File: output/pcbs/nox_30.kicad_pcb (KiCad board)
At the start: 2 copper layers, 111.1 x 91.5 mm, 46 parts

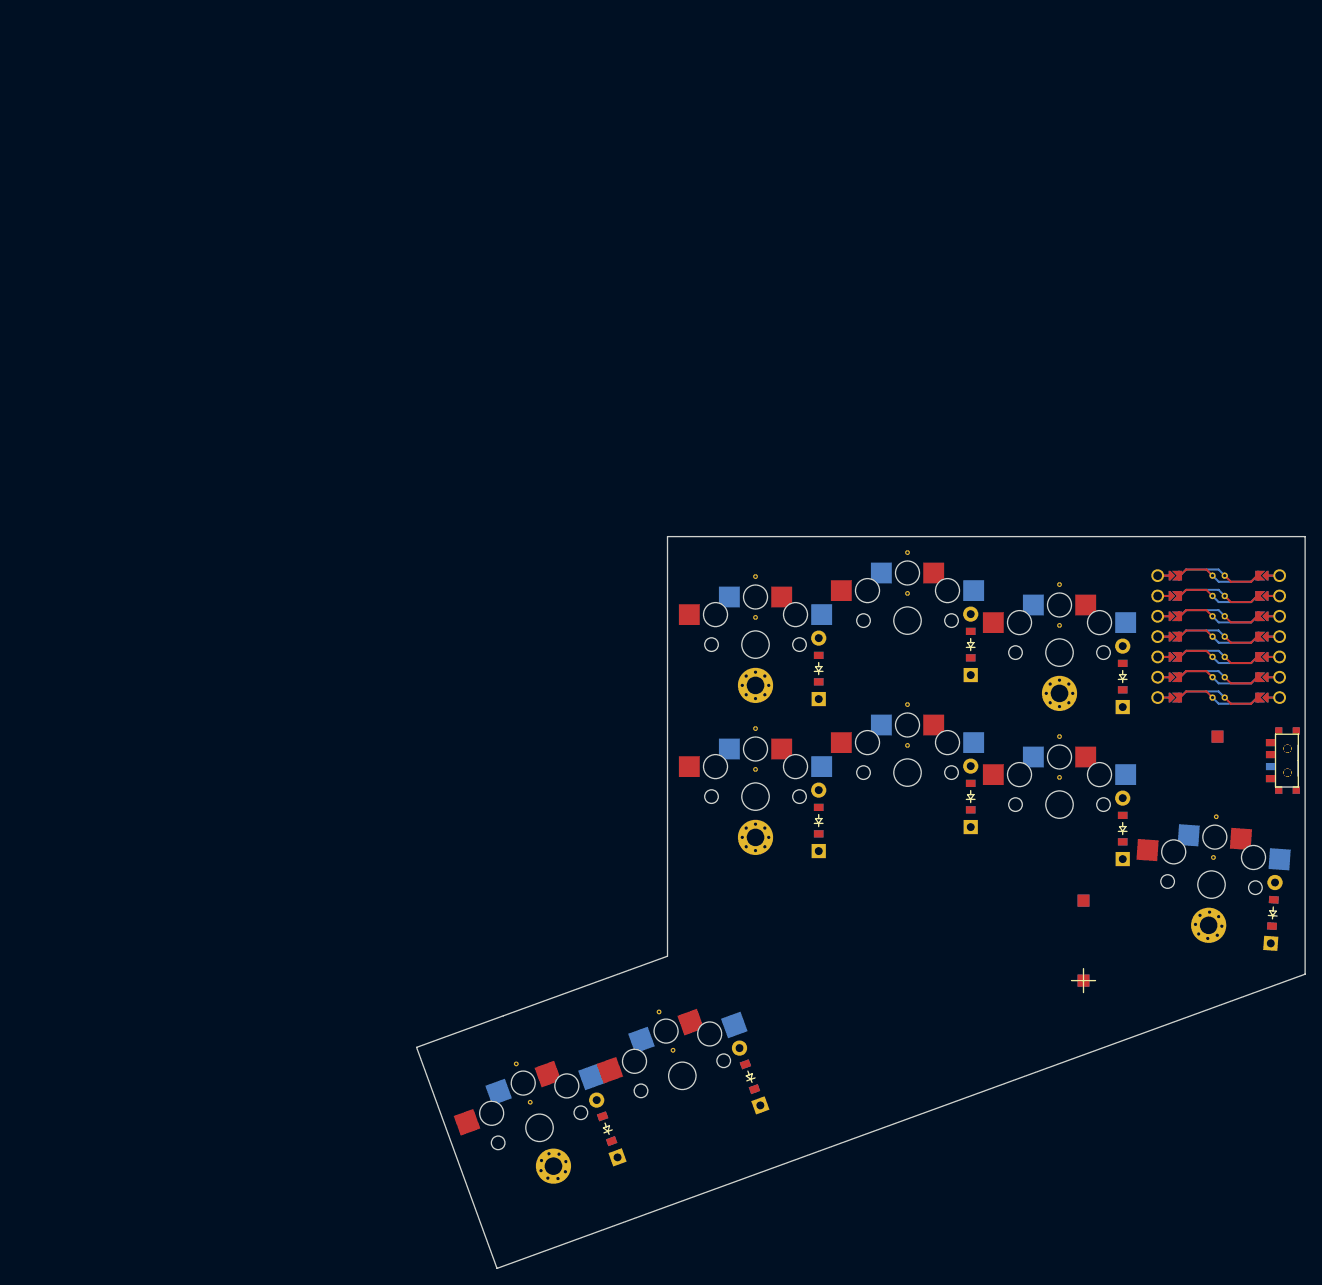
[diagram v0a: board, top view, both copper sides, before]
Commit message: update case
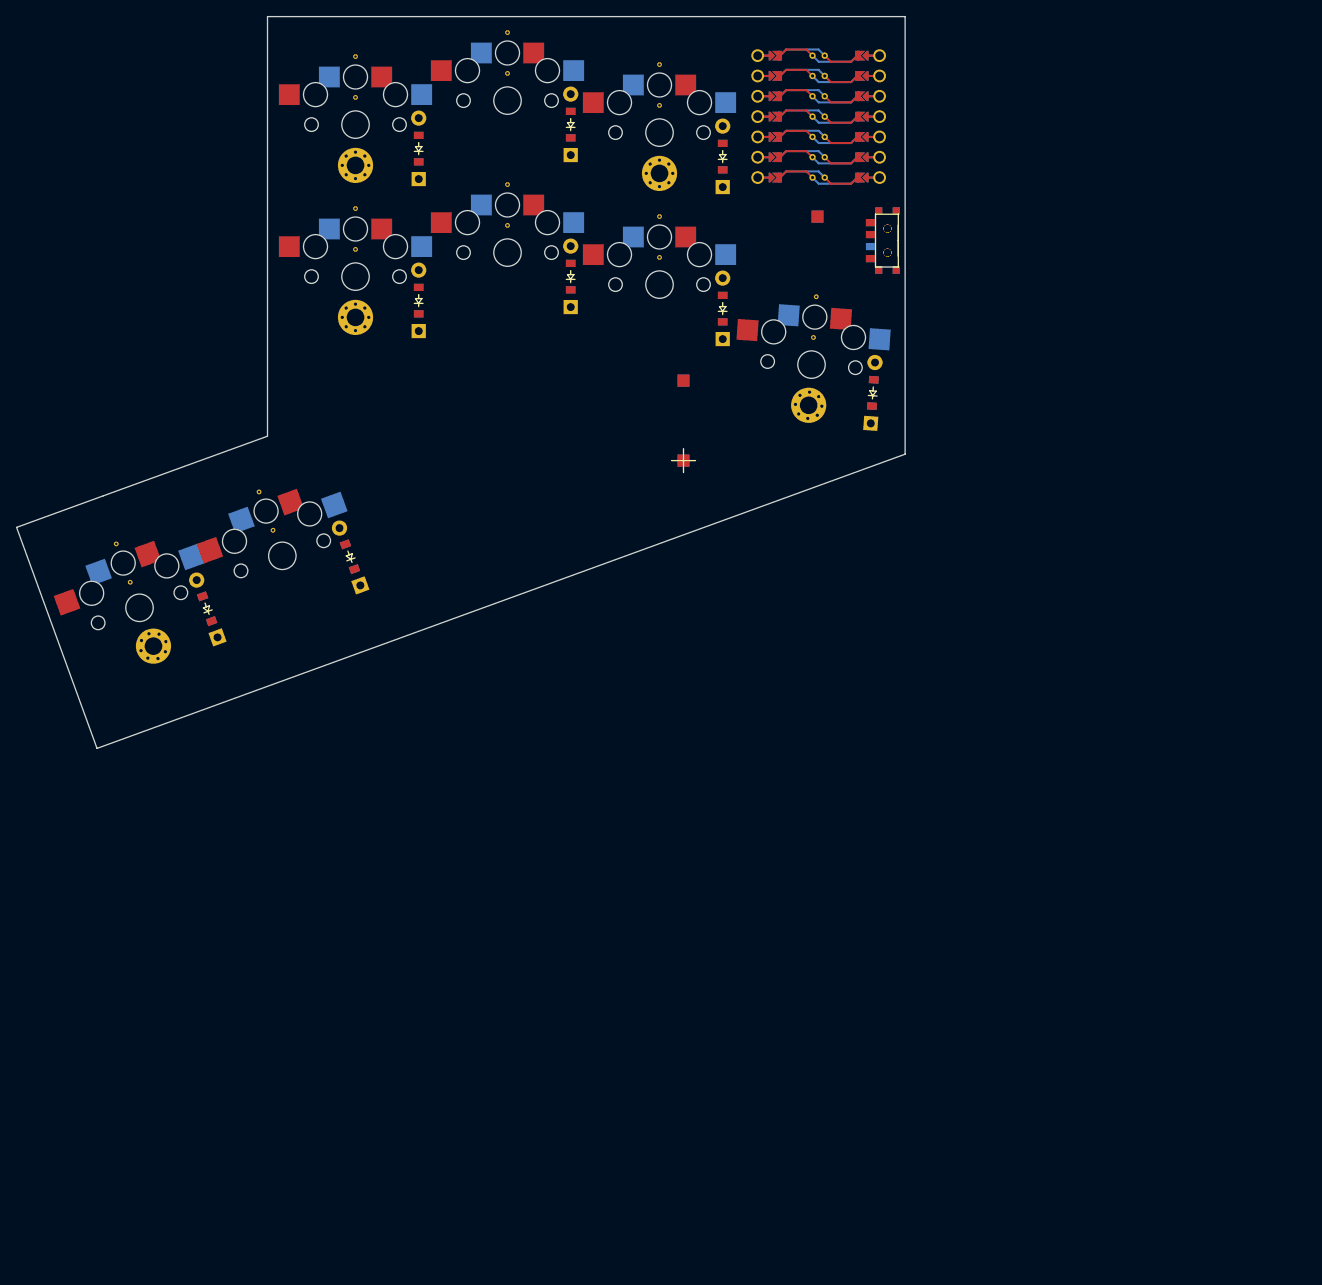
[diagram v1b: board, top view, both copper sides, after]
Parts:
- removed the REF** at (50.0, 62.5)
- removed the REF** at (50.0, 67.6)
- removed the REF** at (50.0, 48.6)
- removed the REF** at (69.0, 64.6)
- removed the REF** at (69.0, 45.6)
- removed the REF** at (88.0, 68.6)
- removed the REF** at (88.0, 49.6)
- removed the REF** at (107.2, 78.6)
- removed the REF** at (21.8, 109.2)
- removed the REF** at (39.7, 102.7)
- removed the REF** at (50.0, 43.5)
- removed the REF** at (69.0, 59.5)
- removed the REF** at (69.0, 40.5)
- removed the REF** at (88.0, 63.5)
- removed the REF** at (88.0, 44.5)
- removed the REF** at (107.6, 73.5)
- removed the REF** at (20.1, 104.4)
- removed the REF** at (37.9, 97.9)
- added REF**: VIA-0.6mm, VIA-0.6mm, F.Cu at (0.00, -2.50)
- added REF**: VIA-0.6mm, VIA-0.6mm, F.Cu at (0.00, 2.60)
- added REF**: VIA-0.6mm, VIA-0.6mm, F.Cu at (0.00, -16.4)
- added REF**: VIA-0.6mm, VIA-0.6mm, F.Cu at (19.0, -0.40)
- added REF**: VIA-0.6mm, VIA-0.6mm, F.Cu at (19.0, -19.4)
- added REF**: VIA-0.6mm, VIA-0.6mm, F.Cu at (38.0, 3.60)
- added REF**: VIA-0.6mm, VIA-0.6mm, F.Cu at (38.0, -15.4)
- added REF**: VIA-0.6mm, VIA-0.6mm, F.Cu at (57.2, 13.6)
- added REF**: VIA-0.6mm, VIA-0.6mm, F.Cu at (-28.2, 44.2)
- added REF**: VIA-0.6mm, VIA-0.6mm, F.Cu at (-10.3, 37.7)
- added REF**: VIA-0.6mm, VIA-0.6mm, F.Cu at (0.00, -21.5)
- added REF**: VIA-0.6mm, VIA-0.6mm, F.Cu at (19.0, -5.50)
- added REF**: VIA-0.6mm, VIA-0.6mm, F.Cu at (19.0, -24.5)
- added REF**: VIA-0.6mm, VIA-0.6mm, F.Cu at (38.0, -1.50)
- added REF**: VIA-0.6mm, VIA-0.6mm, F.Cu at (38.0, -20.5)
- added REF**: VIA-0.6mm, VIA-0.6mm, F.Cu at (57.6, 8.52)
- added REF**: VIA-0.6mm, VIA-0.6mm, F.Cu at (-29.9, 39.4)
- added REF**: VIA-0.6mm, VIA-0.6mm, F.Cu at (-12.1, 32.9)
- moved D9 82.0 mm to (-0.70, 41.0)
- moved D3 82.0 mm to (26.9, 6.00)
- moved D4 82.0 mm to (26.9, -13.0)
- moved D5 82.0 mm to (45.9, 10.0)
- moved D6 82.0 mm to (45.9, -9.00)
- moved D8 82.0 mm to (-18.6, 47.5)
- moved S9 82.0 mm to (-9.15, 40.9)
- moved _22 82.0 mm to (56.6, 22.1)
- moved BATTPAD1 82.0 mm to (41.0, 24.0)
- moved D1 82.0 mm to (7.90, 9.00)
- moved D2 82.0 mm to (7.90, -10.0)
- moved D7 82.0 mm to (64.7, 20.5)
- moved PAD1 82.0 mm to (57.8, -1.50)
- moved S1 82.0 mm to (0.00, 6.00)
- moved S2 82.0 mm to (0.00, -13.0)
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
